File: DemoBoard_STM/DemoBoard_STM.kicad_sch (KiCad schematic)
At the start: 60 parts, among them J1 USB4110GFA, J2 Conn_ST_STDC14, J6 M55-7101242R, J7 MSD-1-A, J8 Conn_01x17_Pin, SW1 SW_Push, SW2 SW_Push, U1 STM32U375CGT6Q, U2 W25Q128JVSIM, U3 MCP2518FDT-E_QBB, U4 TCAN332DCNR, U5 TLV75533PDBVR, Y1 32.768kHz, Y2 ABM8-20.000MHZ-10-B1U-T, Y3 16MHz

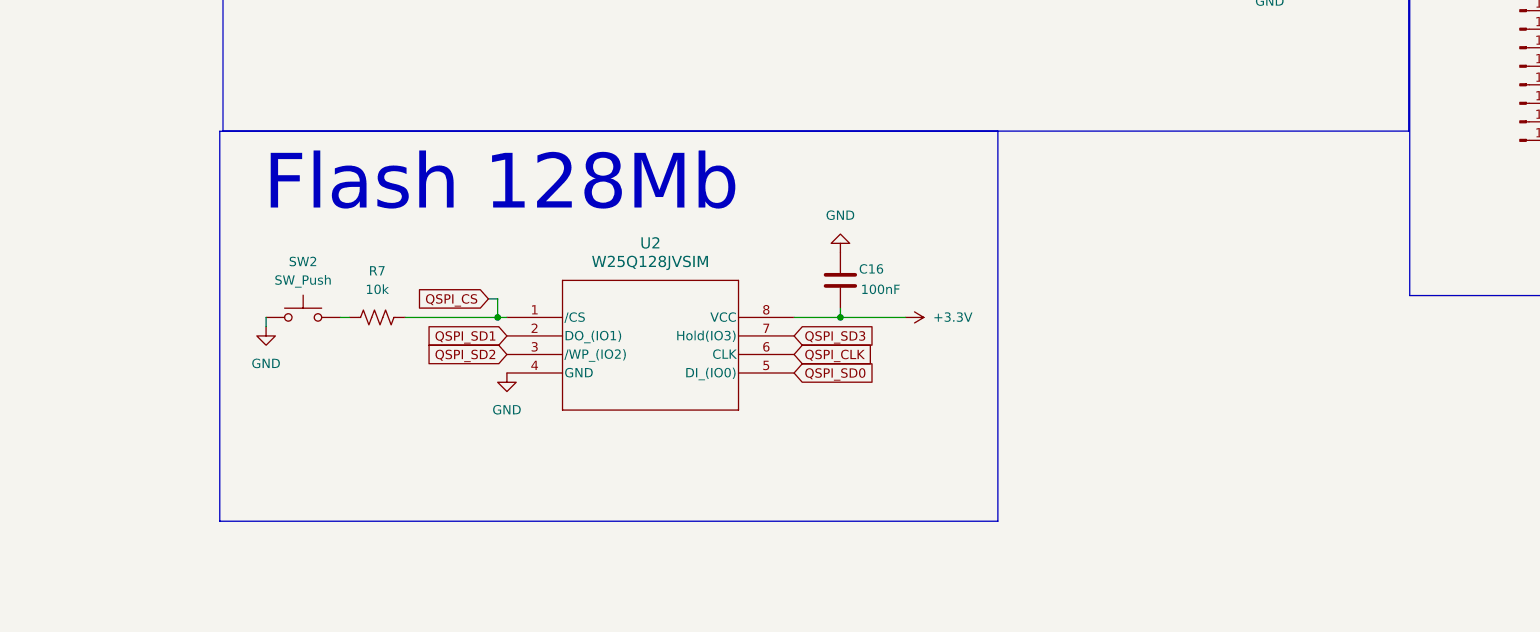
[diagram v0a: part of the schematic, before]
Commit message: added flash
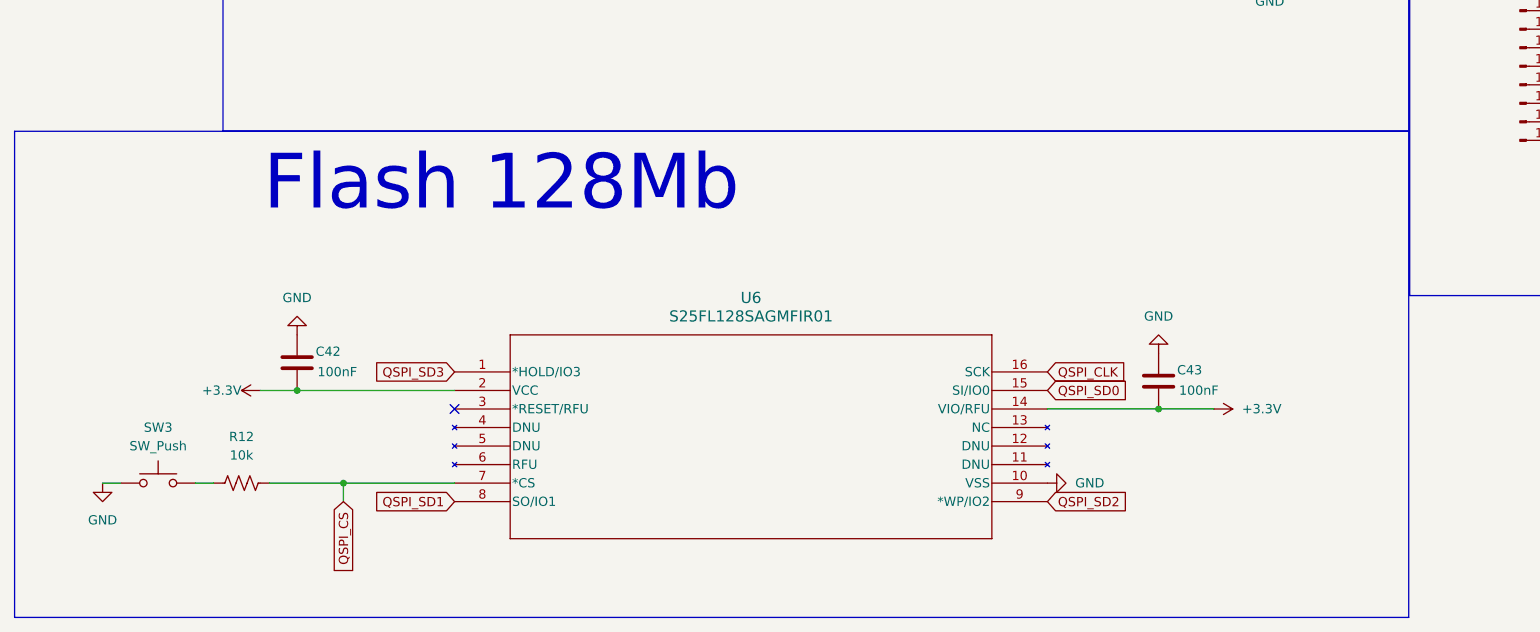
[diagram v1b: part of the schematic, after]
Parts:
- removed C16: 100nF, Capacitor_SMD:C_0402_1005Metric_Pad0.74x0.62mm_HandSolder, symbol Device:C
- removed R7: 10k, Resistor_SMD:R_0402_1005Metric_Pad0.72x0.64mm_HandSolder, symbol Device:R_US
- removed SW2: SW_Push, inspireFly:SW_TL1015AF160QG, symbol Switch:SW_Push
- removed U2: W25Q128JVSIM, inspireFly:SOIC_128JVSIM_WIN, symbol inspireFly:W25Q128JVSIM
- added C42, C43: 100nF, Capacitor_SMD:C_0402_1005Metric_Pad0.74x0.62mm_HandSolder, symbol Device:C
- added R12: 10k, Resistor_SMD:R_0402_1005Metric_Pad0.72x0.64mm_HandSolder, symbol Device:R_US
- added SW3: SW_Push, inspireFly:SW_TL1015AF160QG, symbol Switch:SW_Push
- added U6: S25FL128SAGMFIR01, SO3016_SPA, symbol S25FL128SAGMFIR01:S25FL128SAGMFIR01
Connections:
- net +3.3V: now also C42.2, C43.2, U6.14 (VIO/RFU), U6.2 (VCC)
- net COVER_GND: now also C42.1, C43.1, SW3.1, U6.10 (VSS)
- net QSPI_CLK: now also U6.16 (SCK)
- net QSPI_CS: now also R12.1, U6.7 (*CS)
- net QSPI_SD0: now also U6.15 (SI/IO0)
- net QSPI_SD1: now also U6.8 (SO/IO1)
- net QSPI_SD2: now also U6.9 (*WP/IO2)
- net QSPI_SD3: now also U6.1 (*HOLD/IO3)
- new net: R12.2, SW3.2
- no-connect marks 8 -> 9
